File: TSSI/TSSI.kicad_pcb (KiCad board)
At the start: 2 copper layers, 86.5 x 62 mm, 65 parts, among them J1 Conn_01x04_Pin, J2 Conn_01x04_Pin, J3 Conn_01x04_Pin, U1 SN74AHC1G02MDCKREP, U2 M74VHC1GT32DFT1G, U3 LM555xN, U5 LM7805_TO220, U6 LED Driver

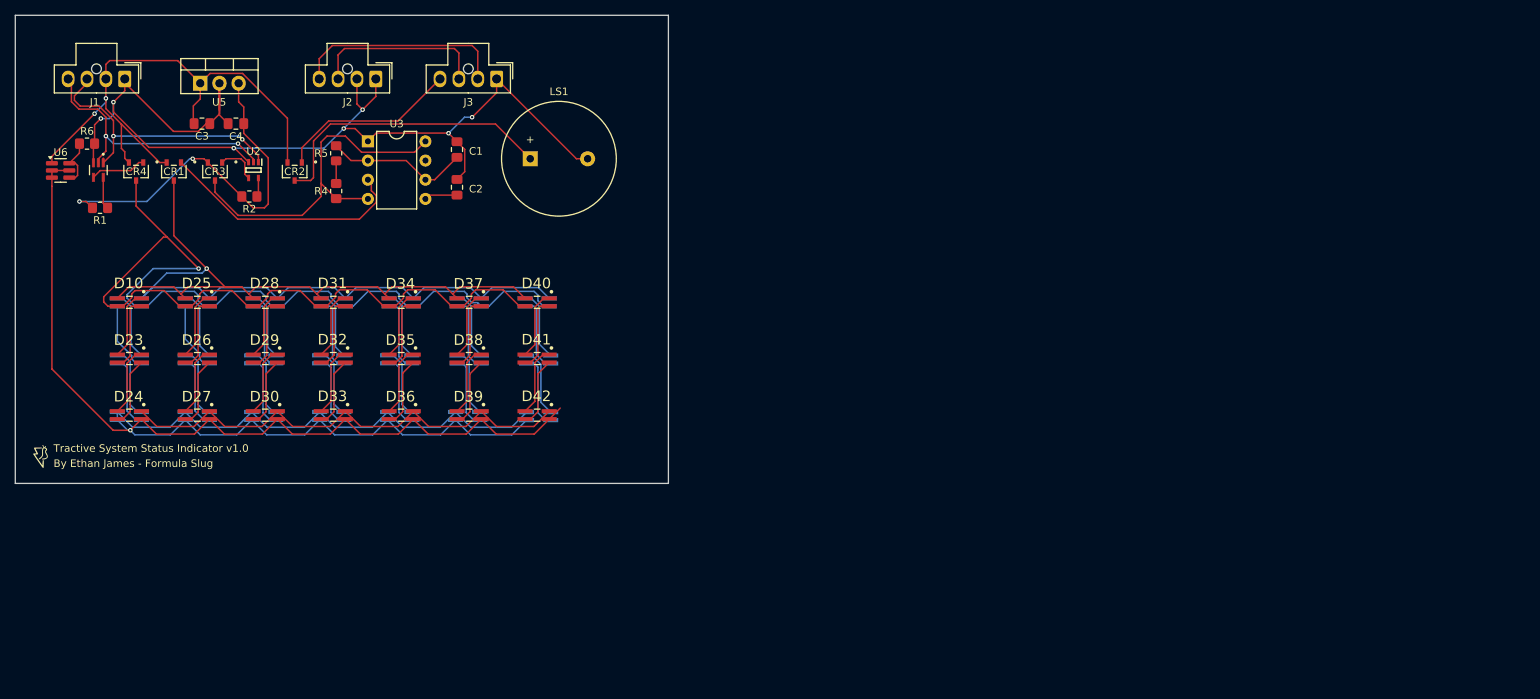
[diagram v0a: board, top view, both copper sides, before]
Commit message: Update Board
new footprints, rearranged board for compactness, adjusted connectors to be horizontal for better enclosure clearance.
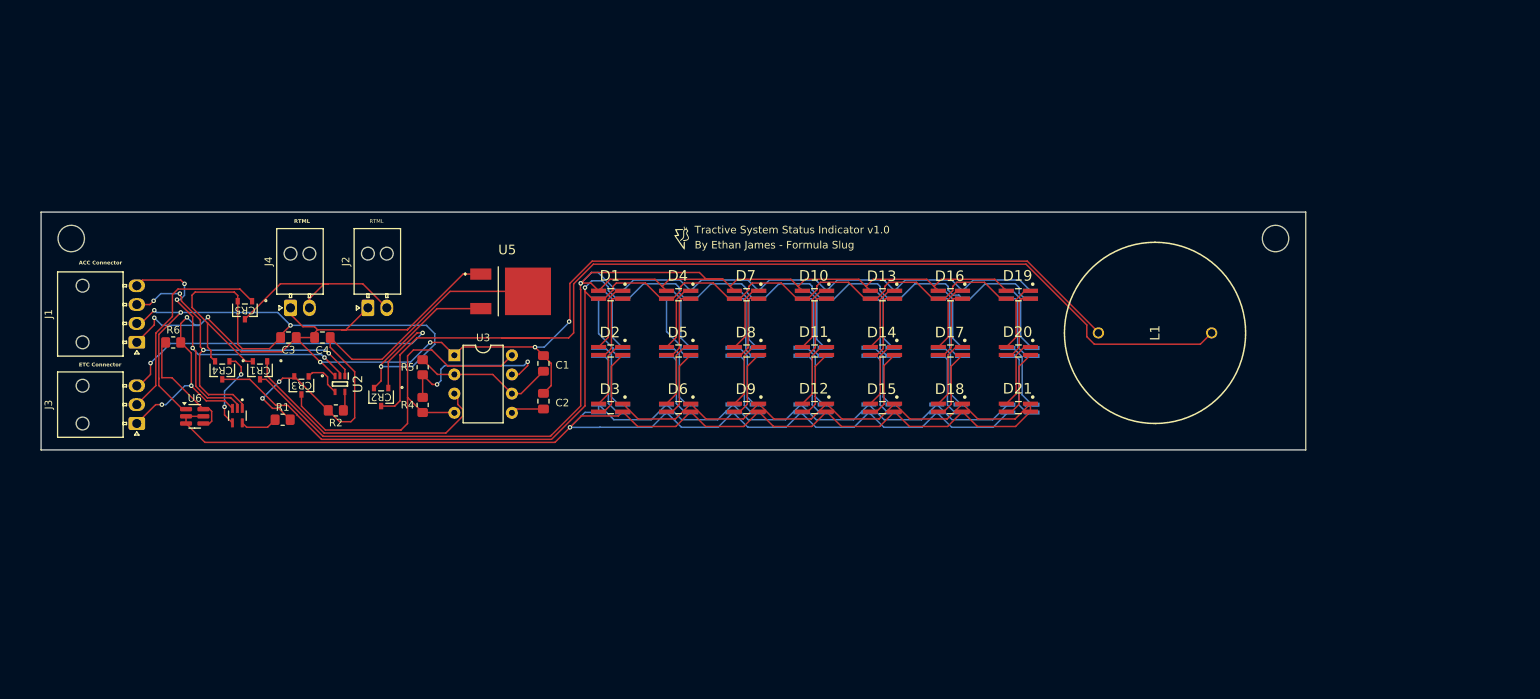
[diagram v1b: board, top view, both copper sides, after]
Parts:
- removed LS1: Speaker, Buzzer_Beeper:Buzzer_15x7.5RM7.6
- added CR5: BSS806NEH6327XTSA1, BSS806NEH6327XTSA1:PG-SOT23-3-5_INF, F.Cu at (59.5, 71.5)
- added J4: Conn_01x02_Pin, Connector_Molex:Molex_Nano-Fit_105313-xx02_1x02_P2.50mm_Horizontal, F.Cu at (65.5, 71.2)
- added L1: PK-21N30PQ, PK-21N20PQ:PK21N30PQ, F.Cu at (187.5, 74.5)
- CR1, CR2, CR3, CR4: footprint footprints:PG-SOT23-3-5_INF -> BSS806NEH6327XTSA1:PG-SOT23-3-5_INF
- D1: renamed from D10; value LED_Dual_AAKK -> XZM2CRKM2DG55W
- D10: renamed from D31; value LED_Dual_AAKK -> XZM2CRKM2DG55W
- D11: renamed from D32; value LED_Dual_AAKK -> XZM2CRKM2DG55W
- D12: renamed from D33; value LED_Dual_AAKK -> XZM2CRKM2DG55W
- D13: renamed from D34; value LED_Dual_AAKK -> XZM2CRKM2DG55W
- D14: renamed from D35; value LED_Dual_AAKK -> XZM2CRKM2DG55W
- D15: renamed from D36; value LED_Dual_AAKK -> XZM2CRKM2DG55W
- D16: renamed from D37; value LED_Dual_AAKK -> XZM2CRKM2DG55W
- D17: renamed from D38; value LED_Dual_AAKK -> XZM2CRKM2DG55W
- D18: renamed from D39; value LED_Dual_AAKK -> XZM2CRKM2DG55W
- D19: renamed from D40; value LED_Dual_AAKK -> XZM2CRKM2DG55W
- D2: renamed from D23; value LED_Dual_AAKK -> XZM2CRKM2DG55W
- D20: renamed from D41; value LED_Dual_AAKK -> XZM2CRKM2DG55W
- D21: renamed from D42; value LED_Dual_AAKK -> XZM2CRKM2DG55W
- D22: renamed from D1; value LED_Dual_AAKK -> XZM2CRKM2DG55W
- D23: renamed from D8; value LED_Dual_AAKK -> XZM2CRKM2DG55W
- D24: renamed from D16; value LED_Dual_AAKK -> XZM2CRKM2DG55W
- D25: renamed from D2; value LED_Dual_AAKK -> XZM2CRKM2DG55W
- D26: renamed from D9; value LED_Dual_AAKK -> XZM2CRKM2DG55W
- D27: renamed from D17; value LED_Dual_AAKK -> XZM2CRKM2DG55W
- D28: renamed from D3; value LED_Dual_AAKK -> XZM2CRKM2DG55W
- D29: renamed from D11; value LED_Dual_AAKK -> XZM2CRKM2DG55W
- D3: renamed from D24; value LED_Dual_AAKK -> XZM2CRKM2DG55W
- D30: renamed from D18; value LED_Dual_AAKK -> XZM2CRKM2DG55W
- D31: renamed from D4; value LED_Dual_AAKK -> XZM2CRKM2DG55W
- D32: renamed from D12; value LED_Dual_AAKK -> XZM2CRKM2DG55W
- D33: renamed from D19; value LED_Dual_AAKK -> XZM2CRKM2DG55W
- D34: renamed from D5; value LED_Dual_AAKK -> XZM2CRKM2DG55W
- D35: renamed from D13; value LED_Dual_AAKK -> XZM2CRKM2DG55W
- D36: renamed from D20; value LED_Dual_AAKK -> XZM2CRKM2DG55W
- D37: renamed from D6; value LED_Dual_AAKK -> XZM2CRKM2DG55W
- D38: renamed from D14; value LED_Dual_AAKK -> XZM2CRKM2DG55W
- D39: renamed from D21; value LED_Dual_AAKK -> XZM2CRKM2DG55W
- D4: renamed from D25; value LED_Dual_AAKK -> XZM2CRKM2DG55W
- D40: renamed from D7; value LED_Dual_AAKK -> XZM2CRKM2DG55W
- D41: renamed from D15; value LED_Dual_AAKK -> XZM2CRKM2DG55W
- D42: renamed from D22; value LED_Dual_AAKK -> XZM2CRKM2DG55W
- D5: renamed from D26; value LED_Dual_AAKK -> XZM2CRKM2DG55W
- D6: renamed from D27; value LED_Dual_AAKK -> XZM2CRKM2DG55W
- D7: renamed from D28; value LED_Dual_AAKK -> XZM2CRKM2DG55W
- D8: renamed from D29; value LED_Dual_AAKK -> XZM2CRKM2DG55W
- D9: renamed from D30; value LED_Dual_AAKK -> XZM2CRKM2DG55W
- J1: footprint Connector_Molex:Molex_Nano-Fit_105309-xx04_1x04_P2.50mm_Vertical -> Connector_Molex:Molex_Nano-Fit_105313-xx04_1x04_P2.50mm_Horizontal
- J2: value Conn_01x04_Pin -> Conn_01x02_Pin; footprint Connector_Molex:Molex_Nano-Fit_105309-xx04_1x04_P2.50mm_Vertical -> Connector_Molex:Molex_Nano-Fit_105313-xx02_1x02_P2.50mm_Horizontal
- J3: footprint Connector_Molex:Molex_Nano-Fit_105309-xx04_1x04_P2.50mm_Vertical -> Connector_Molex:Molex_Nano-Fit_105313-xx03_1x03_P2.50mm_Horizontal
- U2: footprint KiCad:SOT65P210X110-5N -> M74VHC1GT32DFT1G:SOT65P210X110-5N
- U5: value LM7805_TO220 -> LD1086DT50TR; footprint Package_TO_SOT_THT:TO-220-3_Vertical -> LD1086DT50TR:LD1086DT33TR
- moved G*** 89.7 mm to (120.5, 62.0)
- moved J3 66.0 mm to (45.2, 86.5), turned to 180 degrees
- moved D27 63.7 mm to (152.7, 84.5)
- moved D29 63.7 mm to (143.7, 77.0)
- moved D30 63.7 mm to (143.7, 84.5)
- moved D32 63.7 mm to (134.7, 77.0)
- moved D33 63.7 mm to (134.7, 84.5)
- moved D1 63.7 mm to (107.9, 69.4)
- moved D10 63.7 mm to (134.9, 69.4)
- moved D11 63.7 mm to (134.9, 76.9)
- moved D12 63.7 mm to (134.9, 84.4)
- moved D13 63.7 mm to (143.9, 69.4)
- moved D14 63.7 mm to (143.9, 76.9)
- moved D15 63.7 mm to (143.9, 84.4)
- moved D16 63.7 mm to (152.9, 69.4)
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- renumbered U1 to U4
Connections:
- J2 pad 2: GND -> /RTML_12V
- J3 pad 2: /RTML1_12V -> /RTML_5V
- J3 pad 3: /RTML2_12V -> /RTDS_SIGNAL
- U5 pad 1: +12V -> GND
- U5 pad 2: GND -> +5V
- U5 pad 3: +5V -> +12V
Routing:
- net /RTDS_BUZZER: track 39.1 -> 137.3 mm
- net GND: track 142.8 -> 226.0 mm, vias 7 -> 9
- net /RED_LIGHTS: track 153.7 -> 217.9 mm
- net +12V: track 74.2 -> 126.1 mm, vias 2 -> 4
- net /GREEN_LIGHTS: track 175.4 -> 210.3 mm
- net /RTML1_12V: track 28.4 -> 0.00 mm
- net /RTML_5V: track 0.00 -> 28.0 mm
- net /RTDS_SIGNAL: track 24.0 -> 51.3 mm, vias 0 -> 2
- net /RTML_12V: track 0.00 -> 26.5 mm
- net /TO_DRIVER: track 303.7 -> 329.6 mm
- net /RTML2_12V: track 23.2 -> 0.00 mm
- net Net-(U3-DIS): track 3.00 -> 22.6 mm, vias 0 -> 2
- net /IMD_STATUS: track 36.0 -> 50.5 mm, vias 2 -> 4
- net +5V: track 49.9 -> 63.9 mm
- net /BMS_STATUS: track 37.7 -> 48.0 mm, vias 2 -> 4
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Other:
- board size 86.5 x 62 mm -> 167.5 x 31.5 mm
- board text added: "ACC Connector"
- board text added: "ETC Connector"
- board text added: "RTML"

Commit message: finalized board and library changes
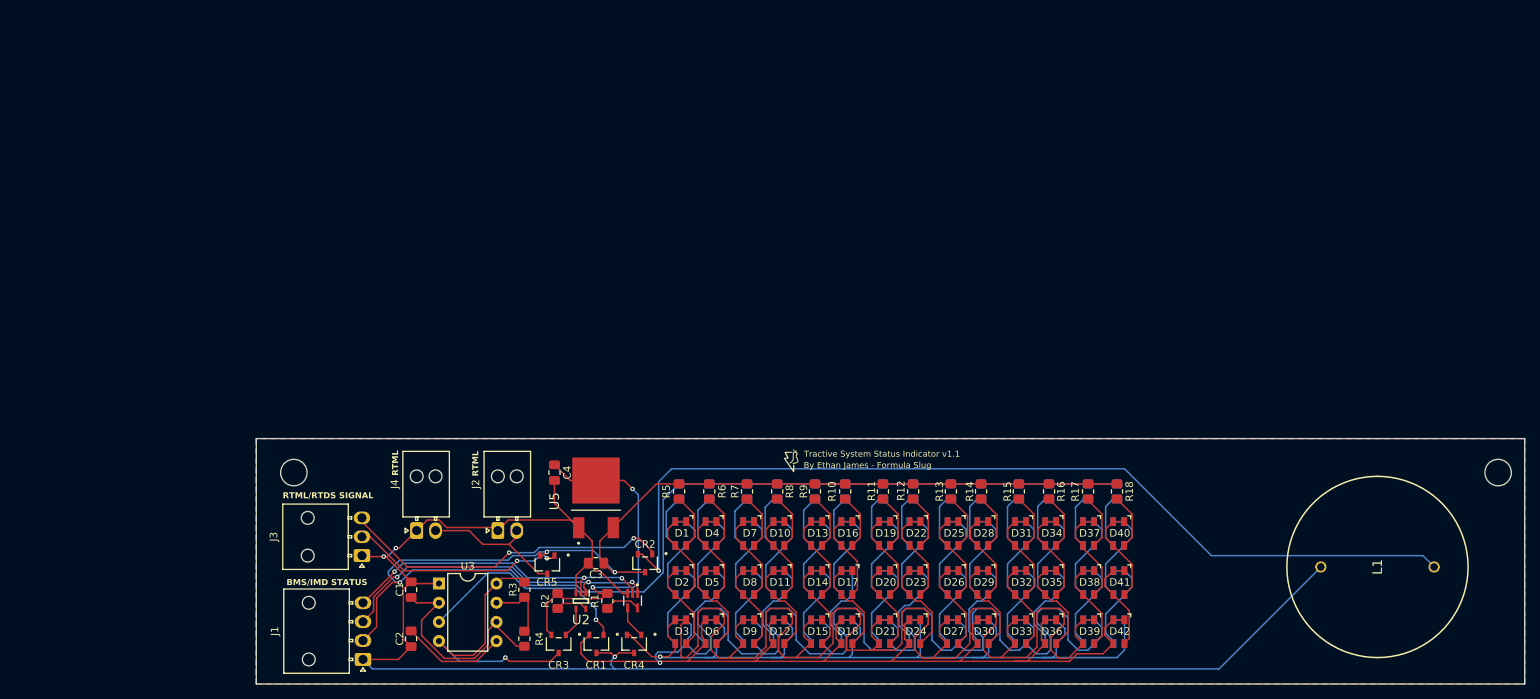
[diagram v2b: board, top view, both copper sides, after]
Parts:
- removed U6: LED Driver, Package_TO_SOT_SMD:SC-74-6_1.55x2.9mm_P0.95mm
- added D43: T1681NG--20C000112U1930, T1681NG--20C000112U1930:T1681NG--20C000112U1930, B.Cu at (175.2, 101.1)
- added D44: T1681NG--20C000112U1930, T1681NG--20C000112U1930:T1681NG--20C000112U1930, B.Cu at (175.3, 107.6)
- added D45: T1681NG--20C000112U1930, T1681NG--20C000112U1930:T1681NG--20C000112U1930, B.Cu at (175.3, 114.1)
- added D46: T1681USD-20C000312U1930, T1681NG--20C000112U1930:T1681NG--20C000112U1930, B.Cu at (171.2, 101.1)
- added D47: T1681USD-20C000312U1930, T1681NG--20C000112U1930:T1681NG--20C000112U1930, B.Cu at (171.3, 107.6)
- added D48: T1681USD-20C000312U1930, T1681NG--20C000112U1930:T1681NG--20C000112U1930, B.Cu at (171.3, 114.1)
- added D49: T1681NG--20C000112U1930, T1681NG--20C000112U1930:T1681NG--20C000112U1930, B.Cu at (166.2, 101.1)
- added D50: T1681NG--20C000112U1930, T1681NG--20C000112U1930:T1681NG--20C000112U1930, B.Cu at (166.2, 107.6)
- added D51: T1681NG--20C000112U1930, T1681NG--20C000112U1930:T1681NG--20C000112U1930, B.Cu at (166.2, 114.1)
- added D52: T1681USD-20C000312U1930, T1681NG--20C000112U1930:T1681NG--20C000112U1930, B.Cu at (162.2, 101.1)
- added D53: T1681USD-20C000312U1930, T1681NG--20C000112U1930:T1681NG--20C000112U1930, B.Cu at (162.3, 107.6)
- added D54: T1681USD-20C000312U1930, T1681NG--20C000112U1930:T1681NG--20C000112U1930, B.Cu at (162.2, 114.1)
- added D55: T1681NG--20C000112U1930, T1681NG--20C000112U1930:T1681NG--20C000112U1930, B.Cu at (157.2, 101.1)
- added D56: T1681NG--20C000112U1930, T1681NG--20C000112U1930:T1681NG--20C000112U1930, B.Cu at (157.2, 107.6)
- added D57: T1681NG--20C000112U1930, T1681NG--20C000112U1930:T1681NG--20C000112U1930, B.Cu at (157.3, 114.1)
- added D58: T1681USD-20C000312U1930, T1681NG--20C000112U1930:T1681NG--20C000112U1930, B.Cu at (153.3, 101.1)
- added D59: T1681USD-20C000312U1930, T1681NG--20C000112U1930:T1681NG--20C000112U1930, B.Cu at (153.3, 107.6)
- added D60: T1681USD-20C000312U1930, T1681NG--20C000112U1930:T1681NG--20C000112U1930, B.Cu at (153.2, 114.1)
- added D61: T1681NG--20C000112U1930, T1681NG--20C000112U1930:T1681NG--20C000112U1930, B.Cu at (148.2, 101.1)
- added D62: T1681NG--20C000112U1930, T1681NG--20C000112U1930:T1681NG--20C000112U1930, B.Cu at (148.2, 107.6)
- added D63: T1681NG--20C000112U1930, T1681NG--20C000112U1930:T1681NG--20C000112U1930, B.Cu at (148.2, 114.1)
- added D64: T1681USD-20C000312U1930, T1681NG--20C000112U1930:T1681NG--20C000112U1930, B.Cu at (144.2, 101.1)
- added D65: T1681USD-20C000312U1930, T1681NG--20C000112U1930:T1681NG--20C000112U1930, B.Cu at (144.2, 107.6)
- added D66: T1681USD-20C000312U1930, T1681NG--20C000112U1930:T1681NG--20C000112U1930, B.Cu at (144.2, 114.1)
- added D67: T1681NG--20C000112U1930, T1681NG--20C000112U1930:T1681NG--20C000112U1930, B.Cu at (139.2, 101.1)
- added D68: T1681NG--20C000112U1930, T1681NG--20C000112U1930:T1681NG--20C000112U1930, B.Cu at (139.2, 107.6)
- added D69: T1681NG--20C000112U1930, T1681NG--20C000112U1930:T1681NG--20C000112U1930, B.Cu at (139.2, 114.1)
- added D70: T1681USD-20C000312U1930, T1681NG--20C000112U1930:T1681NG--20C000112U1930, B.Cu at (135.2, 101.1)
- added D71: T1681USD-20C000312U1930, T1681NG--20C000112U1930:T1681NG--20C000112U1930, B.Cu at (135.2, 107.6)
- added D72: T1681USD-20C000312U1930, T1681NG--20C000112U1930:T1681NG--20C000112U1930, B.Cu at (135.2, 114.1)
- added D73: T1681NG--20C000112U1930, T1681NG--20C000112U1930:T1681NG--20C000112U1930, B.Cu at (130.2, 101.1)
- added D74: T1681NG--20C000112U1930, T1681NG--20C000112U1930:T1681NG--20C000112U1930, B.Cu at (130.2, 107.6)
- added D75: T1681NG--20C000112U1930, T1681NG--20C000112U1930:T1681NG--20C000112U1930, B.Cu at (130.2, 114.1)
- added D76: T1681USD-20C000312U1930, T1681NG--20C000112U1930:T1681NG--20C000112U1930, B.Cu at (126.2, 101.1)
- added D77: T1681USD-20C000312U1930, T1681NG--20C000112U1930:T1681NG--20C000112U1930, B.Cu at (126.2, 107.6)
- added D78: T1681USD-20C000312U1930, T1681NG--20C000112U1930:T1681NG--20C000112U1930, B.Cu at (126.2, 114.1)
- added D79: T1681NG--20C000112U1930, T1681NG--20C000112U1930:T1681NG--20C000112U1930, B.Cu at (121.2, 101.1)
- added D80: T1681NG--20C000112U1930, T1681NG--20C000112U1930:T1681NG--20C000112U1930, B.Cu at (121.2, 107.6)
- added D81: T1681NG--20C000112U1930, T1681NG--20C000112U1930:T1681NG--20C000112U1930, B.Cu at (121.2, 114.1)
- added D82: T1681USD-20C000312U1930, T1681NG--20C000112U1930:T1681NG--20C000112U1930, B.Cu at (117.2, 101.1)
- added D83: T1681USD-20C000312U1930, T1681NG--20C000112U1930:T1681NG--20C000112U1930, B.Cu at (117.3, 107.6)
- added D84: T1681USD-20C000312U1930, T1681NG--20C000112U1930:T1681NG--20C000112U1930, B.Cu at (117.2, 114.1)
- added R10: 480, Resistor_SMD:R_0805_2012Metric_Pad1.20x1.40mm_HandSolder, F.Cu at (139.0, 95.5)
- added R11: 330, Resistor_SMD:R_0805_2012Metric_Pad1.20x1.40mm_HandSolder, F.Cu at (144.0, 95.5)
- added R12: 480, Resistor_SMD:R_0805_2012Metric_Pad1.20x1.40mm_HandSolder, F.Cu at (148.0, 95.5)
- added R13: 330, Resistor_SMD:R_0805_2012Metric_Pad1.20x1.40mm_HandSolder, F.Cu at (153.0, 95.5)
- added R14: 480, Resistor_SMD:R_0805_2012Metric_Pad1.20x1.40mm_HandSolder, F.Cu at (157.0, 95.5)
- added R15: 330, Resistor_SMD:R_0805_2012Metric_Pad1.20x1.40mm_HandSolder, F.Cu at (162.0, 95.5)
- added R16: 480, Resistor_SMD:R_0805_2012Metric_Pad1.20x1.40mm_HandSolder, F.Cu at (166.0, 95.5)
- added R17: 330, Resistor_SMD:R_0805_2012Metric_Pad1.20x1.40mm_HandSolder, F.Cu at (171.2, 95.5)
- added R18: 480, Resistor_SMD:R_0805_2012Metric_Pad1.20x1.40mm_HandSolder, F.Cu at (175.0, 95.5)
- added R19: 330, Resistor_SMD:R_0805_2012Metric_Pad1.20x1.40mm_HandSolder, B.Cu at (175.0, 95.5)
- added R20: 480, Resistor_SMD:R_0805_2012Metric_Pad1.20x1.40mm_HandSolder, B.Cu at (171.2, 95.5)
- added R21: 330, Resistor_SMD:R_0805_2012Metric_Pad1.20x1.40mm_HandSolder, B.Cu at (166.0, 95.5)
- added R22: 480, Resistor_SMD:R_0805_2012Metric_Pad1.20x1.40mm_HandSolder, B.Cu at (162.0, 95.5)
- added R23: 330, Resistor_SMD:R_0805_2012Metric_Pad1.20x1.40mm_HandSolder, B.Cu at (157.0, 95.5)
- added R24: 480, Resistor_SMD:R_0805_2012Metric_Pad1.20x1.40mm_HandSolder, B.Cu at (153.0, 95.5)
- added R25: 330, Resistor_SMD:R_0805_2012Metric_Pad1.20x1.40mm_HandSolder, B.Cu at (148.0, 95.5)
- added R26: 480, Resistor_SMD:R_0805_2012Metric_Pad1.20x1.40mm_HandSolder, B.Cu at (144.0, 95.5)
- added R27: 330, Resistor_SMD:R_0805_2012Metric_Pad1.20x1.40mm_HandSolder, B.Cu at (139.0, 95.5)
- added R28: 480, Resistor_SMD:R_0805_2012Metric_Pad1.20x1.40mm_HandSolder, B.Cu at (135.0, 95.5)
- added R29: 330, Resistor_SMD:R_0805_2012Metric_Pad1.20x1.40mm_HandSolder, B.Cu at (130.0, 95.5)
- added R3: 1k, Resistor_SMD:R_0805_2012Metric_Pad1.20x1.40mm_HandSolder, F.Cu at (96.5, 108.5)
- added R30: 480, Resistor_SMD:R_0805_2012Metric_Pad1.20x1.40mm_HandSolder, B.Cu at (126.0, 95.5)
- added R31: 330, Resistor_SMD:R_0805_2012Metric_Pad1.20x1.40mm_HandSolder, B.Cu at (121.0, 95.5)
- added R32: 480, Resistor_SMD:R_0805_2012Metric_Pad1.20x1.40mm_HandSolder, B.Cu at (117.0, 95.5)
- added R7: 330, Resistor_SMD:R_0805_2012Metric_Pad1.20x1.40mm_HandSolder, F.Cu at (126.0, 95.5)
- added R8: 480, Resistor_SMD:R_0805_2012Metric_Pad1.20x1.40mm_HandSolder, F.Cu at (130.0, 95.5)
- added R9: 330, Resistor_SMD:R_0805_2012Metric_Pad1.20x1.40mm_HandSolder, F.Cu at (135.0, 95.5)
- D1, D13, D14, D15, D19, D2, D20, D21, D3, D7, D8, D9: value XZM2CRKM2DG55W -> T1681NG--20C000112U1930; footprint XZM2CRKM2DG55W_8:LED_XZM2CRKM2DG55W-8 -> T1681NG--20C000112U1930:T1681NG--20C000112U1930
- D10, D11, D12, D16, D17, D18, D4, D5, D6: value XZM2CRKM2DG55W -> T1681USD-20C000312U1930; footprint XZM2CRKM2DG55W_8:LED_XZM2CRKM2DG55W-8 -> T1681NG--20C000112U1930:T1681NG--20C000112U1930
- D22, D23, D24, D28, D29, D30, D34, D35, D36, D40, D41, D42: value XZM2CRKM2DG55W -> T1681USD-20C000312U1930; footprint XZM2CRKM2DG55W_8:LED_XZM2CRKM2DG55W-8 -> T1681NG--20C000112U1930:T1681NG--20C000112U1930; moved to F.Cu
- D25, D26, D27, D31, D32, D33, D37, D38, D39: value XZM2CRKM2DG55W -> T1681NG--20C000112U1930; footprint XZM2CRKM2DG55W_8:LED_XZM2CRKM2DG55W-8 -> T1681NG--20C000112U1930:T1681NG--20C000112U1930; moved to F.Cu
- J3: value Conn_01x04_Pin -> Conn_01x03_Pin
- R4: value 1k -> 10k
- R5: value 10k -> 330
- R6: value 100 -> 480
- moved D40 74.3 mm to (175.2, 101.1), turned to 0 degrees
- moved D41 73.9 mm to (175.2, 107.6), turned to 0 degrees
- moved R6 73.7 mm to (121.0, 95.5), turned to -90 degrees
- moved D42 73.5 mm to (175.2, 114.1), turned to 0 degrees
- moved CR4 65.5 mm to (111.0, 115.7)
- moved D37 62.8 mm to (171.2, 101.1), turned to 0 degrees
- moved D38 62.3 mm to (171.2, 107.6), turned to 0 degrees
- moved D39 61.8 mm to (171.2, 114.1), turned to 0 degrees
- moved U4 57.8 mm to (110.8, 110.0)
- moved CR1 57.4 mm to (106.0, 115.7)
- moved CR5 52.3 mm to (99.5, 105.2)
- moved J1 51.6 mm to (75.1, 117.8)
- moved D34 51.2 mm to (166.2, 101.1), turned to 0 degrees
- moved D35 50.7 mm to (166.2, 107.6), turned to 0 degrees
- moved C3 50.5 mm to (106.0, 105.0), turned to 180 degrees
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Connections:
- CR1 pad 2: +12V -> /RED_LIGHTS
- CR1 pad 3: /RED_LIGHTS -> GND
- CR2 pad 2: +12V -> /RTDS_BUZZER
- CR2 pad 3: /RTDS_BUZZER -> +12V
- CR4 pad 2: +12V -> /GREEN_LIGHTS
- CR4 pad 3: /GREEN_LIGHTS -> GND
- D1 pad 1: Net-(D1-K1) -> Net-(D2-A)
- D1 pad 2: /RED_LIGHTS -> Net-(D2-A)
- D1 pad 3: Net-(D1-K2) -> Net-(D2-A)
- D1 pad 4: /GREEN_LIGHTS -> Net-(D1-A)
- D10 pad 1: Net-(D10-K1) -> Net-(D11-A)
- D10 pad 2: /RED_LIGHTS -> Net-(D11-A)
- D10 pad 3: Net-(D10-K2) -> Net-(D11-A)
- D10 pad 4: /GREEN_LIGHTS -> Net-(D10-A)
- D11 pad 1: Net-(D11-K1) -> Net-(D12-A)
- D11 pad 2: Net-(D10-K1) -> Net-(D12-A)
- D11 pad 3: Net-(D11-K2) -> Net-(D12-A)
- D11 pad 4: Net-(D10-K2) -> Net-(D11-A)
- D12 pad 1: /TO_DRIVER -> /RED_LIGHTS
- D12 pad 2: Net-(D11-K1) -> /RED_LIGHTS
- D12 pad 3: /TO_DRIVER -> /RED_LIGHTS
- D12 pad 4: Net-(D11-K2) -> Net-(D12-A)
- D13 pad 1: Net-(D13-K1) -> Net-(D14-A)
- D13 pad 2: /RED_LIGHTS -> Net-(D14-A)
- D13 pad 3: Net-(D13-K2) -> Net-(D14-A)
- D13 pad 4: /GREEN_LIGHTS -> Net-(D13-A)
- D14 pad 1: Net-(D14-K1) -> Net-(D15-A)
- D14 pad 2: Net-(D13-K1) -> Net-(D15-A)
- D14 pad 3: Net-(D14-K2) -> Net-(D15-A)
- D14 pad 4: Net-(D13-K2) -> Net-(D14-A)
- D15 pad 1: /TO_DRIVER -> /GREEN_LIGHTS
- D15 pad 2: Net-(D14-K1) -> /GREEN_LIGHTS
- D15 pad 3: /TO_DRIVER -> /GREEN_LIGHTS
- D15 pad 4: Net-(D14-K2) -> Net-(D15-A)
- D16 pad 1: Net-(D16-K1) -> Net-(D17-A)
- D16 pad 2: /RED_LIGHTS -> Net-(D17-A)
- D16 pad 3: Net-(D16-K2) -> Net-(D17-A)
- D16 pad 4: /GREEN_LIGHTS -> Net-(D16-A)
- D17 pad 1: Net-(D17-K1) -> Net-(D18-A)
- D17 pad 2: Net-(D16-K1) -> Net-(D18-A)
- D17 pad 3: Net-(D17-K2) -> Net-(D18-A)
- D17 pad 4: Net-(D16-K2) -> Net-(D17-A)
- D18 pad 1: /TO_DRIVER -> /RED_LIGHTS
- D18 pad 2: Net-(D17-K1) -> /RED_LIGHTS
- D18 pad 3: /TO_DRIVER -> /RED_LIGHTS
- D18 pad 4: Net-(D17-K2) -> Net-(D18-A)
- D19 pad 1: Net-(D19-K1) -> Net-(D20-A)
- D19 pad 2: /RED_LIGHTS -> Net-(D20-A)
- D19 pad 3: Net-(D19-K2) -> Net-(D20-A)
- D19 pad 4: /GREEN_LIGHTS -> Net-(D19-A)
- D2 pad 1: Net-(D2-K1) -> Net-(D3-A)
- D2 pad 2: Net-(D1-K1) -> Net-(D3-A)
- D2 pad 3: Net-(D2-K2) -> Net-(D3-A)
- D2 pad 4: Net-(D1-K2) -> Net-(D2-A)
- D20 pad 1: Net-(D20-K1) -> Net-(D21-A)
- D20 pad 2: Net-(D19-K1) -> Net-(D21-A)
- D20 pad 3: Net-(D20-K2) -> Net-(D21-A)
- D20 pad 4: Net-(D19-K2) -> Net-(D20-A)
- D21 pad 1: /TO_DRIVER -> /GREEN_LIGHTS
- D21 pad 2: Net-(D20-K1) -> /GREEN_LIGHTS
- D21 pad 3: /TO_DRIVER -> /GREEN_LIGHTS
- D21 pad 4: Net-(D20-K2) -> Net-(D21-A)
- D22 pad 1: Net-(D22-K1) -> Net-(D23-A)
- D22 pad 2: /RED_LIGHTS -> Net-(D23-A)
- D22 pad 3: Net-(D22-K2) -> Net-(D23-A)
- D22 pad 4: /GREEN_LIGHTS -> Net-(D22-A)
- D23 pad 1: Net-(D23-K1) -> Net-(D24-A)
- D23 pad 2: Net-(D22-K1) -> Net-(D24-A)
- D23 pad 3: Net-(D23-K2) -> Net-(D24-A)
- D23 pad 4: Net-(D22-K2) -> Net-(D23-A)
- D24 pad 1: /TO_DRIVER -> /RED_LIGHTS
- D24 pad 2: Net-(D23-K1) -> /RED_LIGHTS
- D24 pad 3: /TO_DRIVER -> /RED_LIGHTS
- D24 pad 4: Net-(D23-K2) -> Net-(D24-A)
- D25 pad 1: Net-(D25-K1) -> Net-(D26-A)
- D25 pad 2: /RED_LIGHTS -> Net-(D26-A)
- D25 pad 3: Net-(D25-K2) -> Net-(D26-A)
- D25 pad 4: /GREEN_LIGHTS -> Net-(D25-A)
- D26 pad 1: Net-(D26-K1) -> Net-(D27-A)
- D26 pad 2: Net-(D25-K1) -> Net-(D27-A)
- D26 pad 3: Net-(D26-K2) -> Net-(D27-A)
- D26 pad 4: Net-(D25-K2) -> Net-(D26-A)
- D27 pad 1: /TO_DRIVER -> /GREEN_LIGHTS
- D27 pad 2: Net-(D26-K1) -> /GREEN_LIGHTS
- D27 pad 3: /TO_DRIVER -> /GREEN_LIGHTS
- D27 pad 4: Net-(D26-K2) -> Net-(D27-A)
- D28 pad 1: Net-(D28-K1) -> Net-(D29-A)
- D28 pad 2: /RED_LIGHTS -> Net-(D29-A)
- D28 pad 3: Net-(D28-K2) -> Net-(D29-A)
- D28 pad 4: /GREEN_LIGHTS -> Net-(D28-A)
- D29 pad 1: Net-(D29-K1) -> Net-(D30-A)
- D29 pad 2: Net-(D28-K1) -> Net-(D30-A)
- D29 pad 3: Net-(D29-K2) -> Net-(D30-A)
- D29 pad 4: Net-(D28-K2) -> Net-(D29-A)
- D3 pad 1: /TO_DRIVER -> /GREEN_LIGHTS
- D3 pad 2: Net-(D2-K1) -> /GREEN_LIGHTS
- D3 pad 3: /TO_DRIVER -> /GREEN_LIGHTS
- D3 pad 4: Net-(D2-K2) -> Net-(D3-A)
- D30 pad 1: /TO_DRIVER -> /RED_LIGHTS
- D30 pad 2: Net-(D29-K1) -> /RED_LIGHTS
- D30 pad 3: /TO_DRIVER -> /RED_LIGHTS
- D30 pad 4: Net-(D29-K2) -> Net-(D30-A)
- D31 pad 1: Net-(D31-K1) -> Net-(D32-A)
- D31 pad 2: /RED_LIGHTS -> Net-(D32-A)
- D31 pad 3: Net-(D31-K2) -> Net-(D32-A)
- D31 pad 4: /GREEN_LIGHTS -> Net-(D31-A)
- D32 pad 1: Net-(D32-K1) -> Net-(D33-A)
- D32 pad 2: Net-(D31-K1) -> Net-(D33-A)
- D32 pad 3: Net-(D32-K2) -> Net-(D33-A)
- D32 pad 4: Net-(D31-K2) -> Net-(D32-A)
- D33 pad 1: /TO_DRIVER -> /GREEN_LIGHTS
- D33 pad 2: Net-(D32-K1) -> /GREEN_LIGHTS
- D33 pad 3: /TO_DRIVER -> /GREEN_LIGHTS
- D33 pad 4: Net-(D32-K2) -> Net-(D33-A)
- D34 pad 1: Net-(D34-K1) -> Net-(D35-A)
- D34 pad 2: /RED_LIGHTS -> Net-(D35-A)
- D34 pad 3: Net-(D34-K2) -> Net-(D35-A)
- D34 pad 4: /GREEN_LIGHTS -> Net-(D34-A)
- D35 pad 1: Net-(D35-K1) -> Net-(D36-A)
- D35 pad 2: Net-(D34-K1) -> Net-(D36-A)
- D35 pad 3: Net-(D35-K2) -> Net-(D36-A)
- D35 pad 4: Net-(D34-K2) -> Net-(D35-A)
- D36 pad 1: /TO_DRIVER -> /RED_LIGHTS
- D36 pad 2: Net-(D35-K1) -> /RED_LIGHTS
- D36 pad 3: /TO_DRIVER -> /RED_LIGHTS
- D36 pad 4: Net-(D35-K2) -> Net-(D36-A)
- D37 pad 1: Net-(D37-K1) -> Net-(D38-A)
- D37 pad 2: /RED_LIGHTS -> Net-(D38-A)
- D37 pad 3: Net-(D37-K2) -> Net-(D38-A)
- D37 pad 4: /GREEN_LIGHTS -> Net-(D37-A)
- D38 pad 1: Net-(D38-K1) -> Net-(D39-A)
- D38 pad 2: Net-(D37-K1) -> Net-(D39-A)
- D38 pad 3: Net-(D38-K2) -> Net-(D39-A)
- D38 pad 4: Net-(D37-K2) -> Net-(D38-A)
- D39 pad 1: /TO_DRIVER -> /GREEN_LIGHTS
- D39 pad 2: Net-(D38-K1) -> /GREEN_LIGHTS
- D39 pad 3: /TO_DRIVER -> /GREEN_LIGHTS
- D39 pad 4: Net-(D38-K2) -> Net-(D39-A)
- D4 pad 1: Net-(D4-K1) -> Net-(D5-A)
- D4 pad 2: /RED_LIGHTS -> Net-(D5-A)
- D4 pad 3: Net-(D4-K2) -> Net-(D5-A)
- D4 pad 4: /GREEN_LIGHTS -> Net-(D4-A)
- D40 pad 1: Net-(D40-K1) -> Net-(D41-A)
- D40 pad 2: /RED_LIGHTS -> Net-(D41-A)
- D40 pad 3: Net-(D40-K2) -> Net-(D41-A)
- D40 pad 4: /GREEN_LIGHTS -> Net-(D40-A)
- D41 pad 1: Net-(D41-K1) -> Net-(D42-A)
- D41 pad 2: Net-(D40-K1) -> Net-(D42-A)
- D41 pad 3: Net-(D41-K2) -> Net-(D42-A)
- D41 pad 4: Net-(D40-K2) -> Net-(D41-A)
- D42 pad 1: /TO_DRIVER -> /RED_LIGHTS
- D42 pad 2: Net-(D41-K1) -> /RED_LIGHTS
- D42 pad 3: /TO_DRIVER -> /RED_LIGHTS
- D42 pad 4: Net-(D41-K2) -> Net-(D42-A)
- D5 pad 1: Net-(D5-K1) -> Net-(D6-A)
- D5 pad 2: Net-(D4-K1) -> Net-(D6-A)
- D5 pad 3: Net-(D5-K2) -> Net-(D6-A)
- D5 pad 4: Net-(D4-K2) -> Net-(D5-A)
- D6 pad 1: /TO_DRIVER -> /RED_LIGHTS
- D6 pad 2: Net-(D5-K1) -> /RED_LIGHTS
- D6 pad 3: /TO_DRIVER -> /RED_LIGHTS
- D6 pad 4: Net-(D5-K2) -> Net-(D6-A)
- D7 pad 1: Net-(D7-K1) -> Net-(D8-A)
- D7 pad 2: /RED_LIGHTS -> Net-(D8-A)
- D7 pad 3: Net-(D7-K2) -> Net-(D8-A)
- D7 pad 4: /GREEN_LIGHTS -> Net-(D7-A)
- D8 pad 1: Net-(D8-K1) -> Net-(D9-A)
- D8 pad 2: Net-(D7-K1) -> Net-(D9-A)
- D8 pad 3: Net-(D8-K2) -> Net-(D9-A)
- D8 pad 4: Net-(D7-K2) -> Net-(D8-A)
- D9 pad 1: /TO_DRIVER -> /GREEN_LIGHTS
- D9 pad 2: Net-(D8-K1) -> /GREEN_LIGHTS
- D9 pad 3: /TO_DRIVER -> /GREEN_LIGHTS
- D9 pad 4: Net-(D8-K2) -> Net-(D9-A)
- R4 pad 1: /FLASH_ACTIVE -> Net-(U3-DIS)
- R4 pad 2: Net-(U3-DIS) -> Net-(U3-THR)
- R5 pad 1: Net-(U3-DIS) -> +12V
- R5 pad 2: Net-(U3-THR) -> Net-(D1-A)
- R6 pad 1: Net-(U6-GND) -> +12V
- R6 pad 2: GND -> Net-(D4-A)
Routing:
- net /TO_DRIVER: track 329.6 -> 0.00 mm, vias 1 -> 0
- net +12V: track 126.1 -> 235.4 mm, vias 4 -> 3
- net /GREEN_LIGHTS: track 210.3 -> 314.4 mm
- net /RED_LIGHTS: track 217.9 -> 308.3 mm
- net +5V: track 63.9 -> 46.4 mm
- net Net-(U6-GND): track 15.9 -> 0.00 mm
- net Net-(D81-A): track 0.00 -> 14.7 mm
- net Net-(D6-A): track 0.00 -> 14.2 mm
- net Net-(D36-A): track 0.00 -> 14.2 mm
- net Net-(D18-A): track 0.00 -> 14.2 mm
- net Net-(D12-A): track 0.00 -> 14.2 mm
- net Net-(D24-A): track 0.00 -> 14.2 mm
- net Net-(D30-A): track 0.00 -> 14.2 mm
- net Net-(D75-A): track 0.00 -> 14.1 mm
- net Net-(D83-A): track 0.00 -> 14.0 mm
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- added copper zone on B.Cu, net GND
- added copper zone on F.Cu, net GND
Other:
- board size 167.5 x 31.5 mm -> 168 x 32.5 mm
- board text added: "BMS/IMD STATUS"
- board text added: "RTML/RTDS SIGNAL"
- board text added: "Tractive System Status Indicator v1.1"
- board text removed: "ACC Connector"
- board text removed: "ETC Connector"
- board text removed: "Tractive System Status Indicator v1.0"
